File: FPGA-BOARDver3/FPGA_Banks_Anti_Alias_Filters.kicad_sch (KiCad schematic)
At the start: 1 part, among them U1 XC7Z020-1CLG400I__

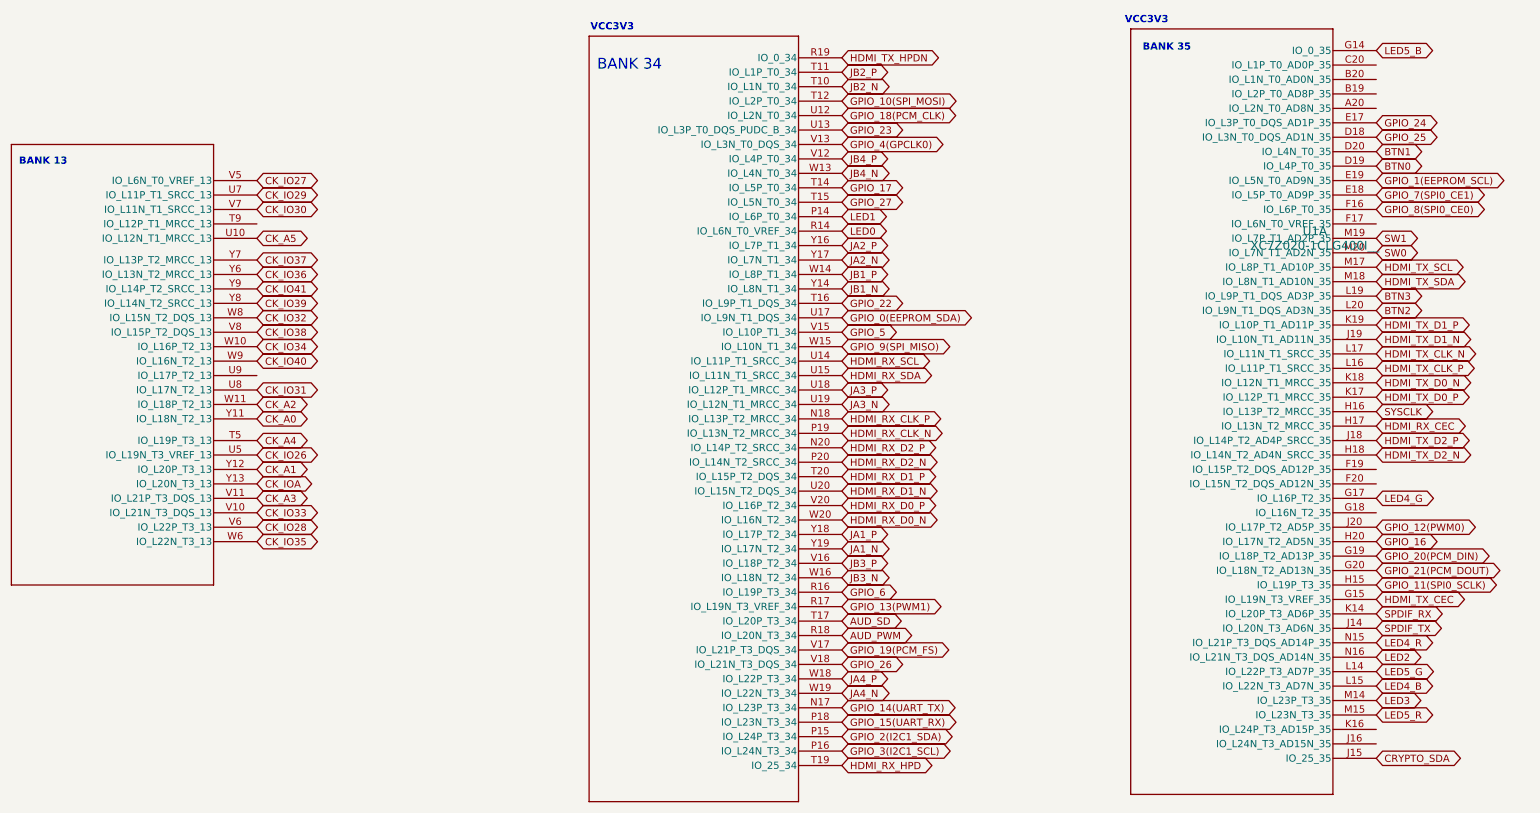
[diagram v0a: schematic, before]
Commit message: updated schematic and layout
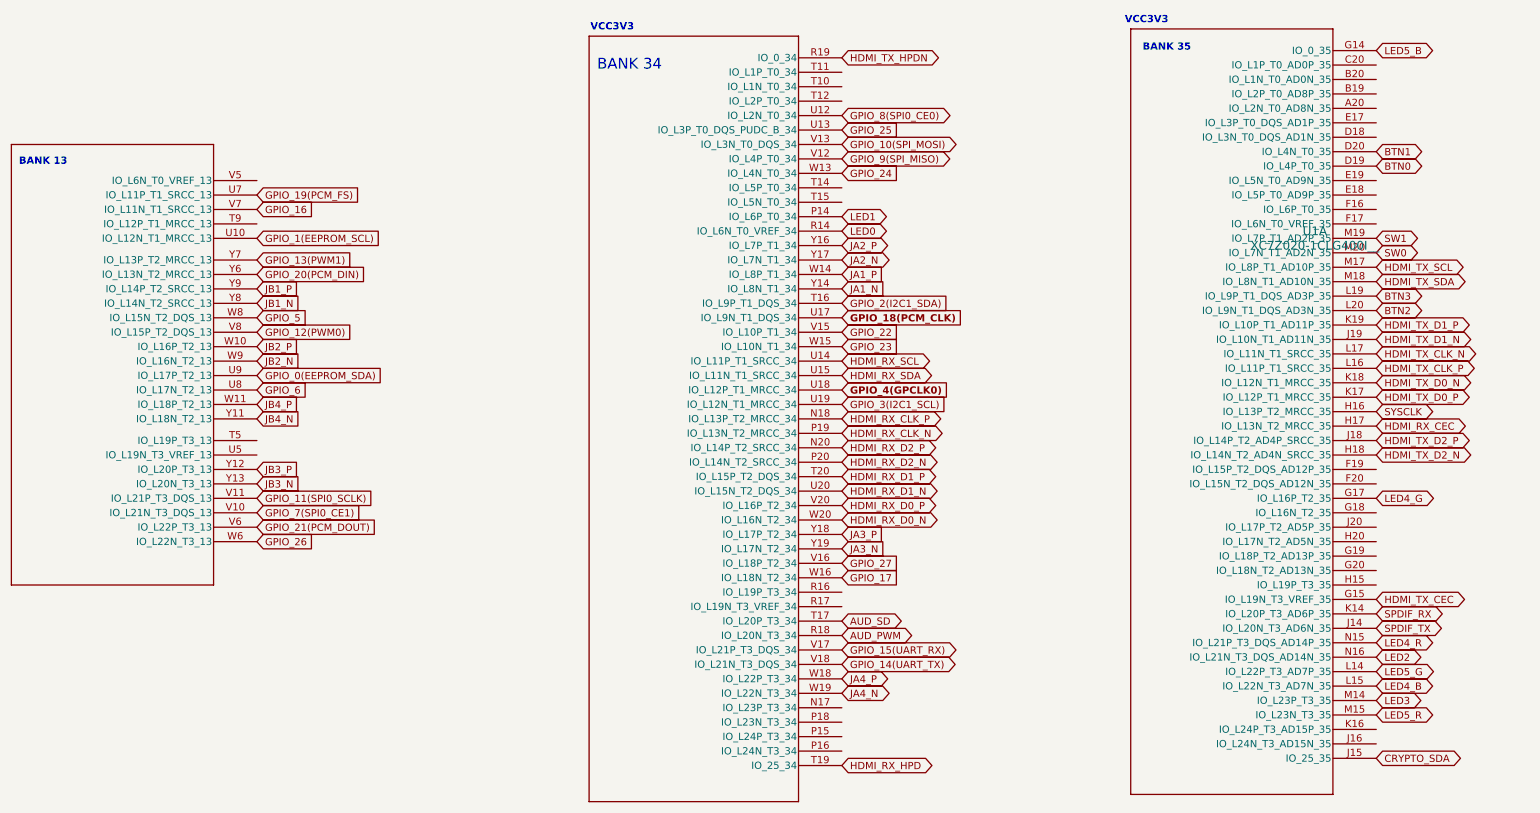
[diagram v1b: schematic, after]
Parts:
- U1: LCSC PN (none) -> C1519081
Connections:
- net CK_A0 is gone; now on net JB4_N: U1.Y11 (IO_L18N_T2_13)
- net CK_A1 is gone; now on net JB3_P: U1.Y12 (IO_L20P_T3_13)
- net CK_A2 is gone; now on net JB4_P: U1.W11 (IO_L18P_T2_13)
- net CK_A3 is gone; now on net GPIO_11(SPI0_SCLK): U1.V11 (IO_L21P_T3_DQS_13)
- net CK_A5 is gone; now on net GPIO_1(EEPROM_SCL): U1.U10 (IO_L12N_T1_MRCC_13)
- net CK_IO28 is gone; now on net GPIO_21(PCM_DOUT): U1.V6 (IO_L22P_T3_13)
- net CK_IO29 is gone; now on net GPIO_19(PCM_FS): U1.U7 (IO_L11P_T1_SRCC_13)
- net CK_IO30 is gone; now on net GPIO_16: U1.V7 (IO_L11N_T1_SRCC_13)
- net CK_IO31 is gone; now on net GPIO_6: U1.U8 (IO_L17N_T2_13)
- net CK_IO32 is gone; now on net GPIO_5: U1.W8 (IO_L15N_T2_DQS_13)
- net CK_IO33 is gone; now on net GPIO_7(SPI0_CE1): U1.V10 (IO_L21N_T3_DQS_13)
- net CK_IO34 is gone; now on net JB2_P: U1.W10 (IO_L16P_T2_13)
- net CK_IO35 is gone; now on net GPIO_26: U1.W6 (IO_L22N_T3_13)
- net CK_IO36 is gone; now on net GPIO_20(PCM_DIN): U1.Y6 (IO_L13N_T2_MRCC_13)
- net CK_IO37 is gone; now on net GPIO_13(PWM1): U1.Y7 (IO_L13P_T2_MRCC_13)
- net CK_IO38 is gone; now on net GPIO_12(PWM0): U1.V8 (IO_L15P_T2_DQS_13)
- net CK_IO39 is gone; now on net JB1_N: U1.Y8 (IO_L14N_T2_SRCC_13)
- net CK_IO40 is gone; now on net JB2_N: U1.W9 (IO_L16N_T2_13)
- net CK_IO41 is gone; now on net JB1_P: U1.Y9 (IO_L14P_T2_SRCC_13)
- net CK_IOA is gone; now on net JB3_N: U1.Y13 (IO_L20N_T3_13)
- net GPIO_0(EEPROM_SDA): now also U1.U9 (IO_L17P_T2_13); no longer U1.U17 (IO_L9N_T1_DQS_34)
- net GPIO_1(EEPROM_SCL): no longer U1.E19 (IO_L5N_T0_AD9N_35)
- net GPIO_10(SPI_MOSI): now also U1.V13 (IO_L3N_T0_DQS_34); no longer U1.T12 (IO_L2P_T0_34)
- net GPIO_11(SPI0_SCLK): no longer U1.H15 (IO_L19P_T3_35)
- net GPIO_12(PWM0): no longer U1.J20 (IO_L17P_T2_AD5P_35)
- net GPIO_13(PWM1): no longer U1.R17 (IO_L19N_T3_VREF_34)
- net GPIO_14(UART_TX): now also U1.V18 (IO_L21N_T3_DQS_34); no longer U1.N17 (IO_L23P_T3_34)
- net GPIO_15(UART_RX): now also U1.V17 (IO_L21P_T3_DQS_34); no longer U1.P18 (IO_L23N_T3_34)
- net GPIO_16: no longer U1.H20 (IO_L17N_T2_AD5N_35)
- net GPIO_17: now also U1.W16 (IO_L18N_T2_34); no longer U1.T14 (IO_L5P_T0_34)
- net GPIO_18(PCM_CLK): now also U1.U17 (IO_L9N_T1_DQS_34); no longer U1.U12 (IO_L2N_T0_34)
- net GPIO_19(PCM_FS): no longer U1.V17 (IO_L21P_T3_DQS_34)
- net GPIO_2(I2C1_SDA): now also U1.T16 (IO_L9P_T1_DQS_34); no longer U1.P15 (IO_L24P_T3_34)
- net GPIO_20(PCM_DIN): no longer U1.G19 (IO_L18P_T2_AD13P_35)
- net GPIO_21(PCM_DOUT): no longer U1.G20 (IO_L18N_T2_AD13N_35)
- net GPIO_22: now also U1.V15 (IO_L10P_T1_34); no longer U1.T16 (IO_L9P_T1_DQS_34)
- net GPIO_23: now also U1.W15 (IO_L10N_T1_34); no longer U1.U13 (IO_L3P_T0_DQS_PUDC_B_34)
- net GPIO_24: now also U1.W13 (IO_L4N_T0_34); no longer U1.E17 (IO_L3P_T0_DQS_AD1P_35)
- net GPIO_25: now also U1.U13 (IO_L3P_T0_DQS_PUDC_B_34); no longer U1.D18 (IO_L3N_T0_DQS_AD1N_35)
- net GPIO_26: no longer U1.V18 (IO_L21N_T3_DQS_34)
- net GPIO_27: now also U1.V16 (IO_L18P_T2_34); no longer U1.T15 (IO_L5N_T0_34)
- net GPIO_3(I2C1_SCL): now also U1.U19 (IO_L12N_T1_MRCC_34); no longer U1.P16 (IO_L24N_T3_34)
- net GPIO_4(GPCLK0): now also U1.U18 (IO_L12P_T1_MRCC_34); no longer U1.V13 (IO_L3N_T0_DQS_34)
- net GPIO_5: no longer U1.V15 (IO_L10P_T1_34)
- net GPIO_6: no longer U1.R16 (IO_L19P_T3_34)
- net GPIO_7(SPI0_CE1): no longer U1.E18 (IO_L5P_T0_AD9P_35)
- net GPIO_8(SPI0_CE0): now also U1.U12 (IO_L2N_T0_34); no longer U1.F16 (IO_L6P_T0_35)
- net GPIO_9(SPI_MISO): now also U1.V12 (IO_L4P_T0_34); no longer U1.W15 (IO_L10N_T1_34)
- net JA1_N: now also U1.Y14 (IO_L8N_T1_34); no longer U1.Y19 (IO_L17N_T2_34)
- net JA1_P: now also U1.W14 (IO_L8P_T1_34); no longer U1.Y18 (IO_L17P_T2_34)
- net JA3_N: now also U1.Y19 (IO_L17N_T2_34); no longer U1.U19 (IO_L12N_T1_MRCC_34)
- net JA3_P: now also U1.Y18 (IO_L17P_T2_34); no longer U1.U18 (IO_L12P_T1_MRCC_34)
- net JB1_N: no longer U1.Y14 (IO_L8N_T1_34)
- net JB1_P: no longer U1.W14 (IO_L8P_T1_34)
- net JB2_N: no longer U1.T10 (IO_L1N_T0_34)
- net JB2_P: no longer U1.T11 (IO_L1P_T0_34)
- net JB3_N: no longer U1.W16 (IO_L18N_T2_34)
- net JB3_P: no longer U1.V16 (IO_L18P_T2_34)
- net JB4_N: no longer U1.W13 (IO_L4N_T0_34)
- net JB4_P: no longer U1.V12 (IO_L4P_T0_34)
- net CK_A4: no longer names the net of U1.T5 (IO_L19P_T3_13)
- net CK_IO26: no longer names the net of U1.U5 (IO_L19N_T3_VREF_13)
- net CK_IO27: no longer names the net of U1.V5 (IO_L6N_T0_VREF_13)
